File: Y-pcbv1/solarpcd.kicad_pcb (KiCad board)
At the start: 6 copper layers, 64 x 58 mm, 53 parts, among them IC2 TSL2561, J1 XF2M-1015-1A, J2 U.FL-R-SMT-1, J3 BATTERY CONNECTOR, U1 SWLP.12.B, U2 Value, U4 SW_SPDT

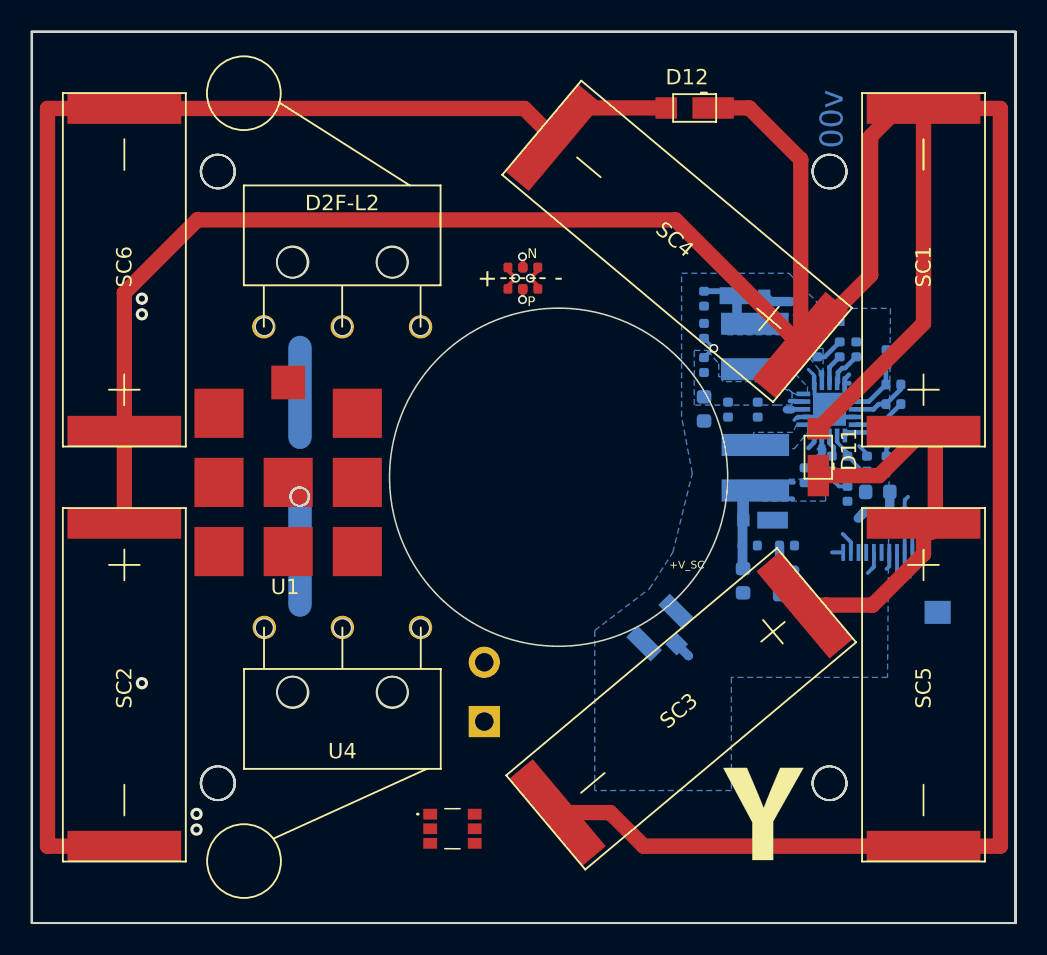
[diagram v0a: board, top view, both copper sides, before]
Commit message: Updated -Y PCB design
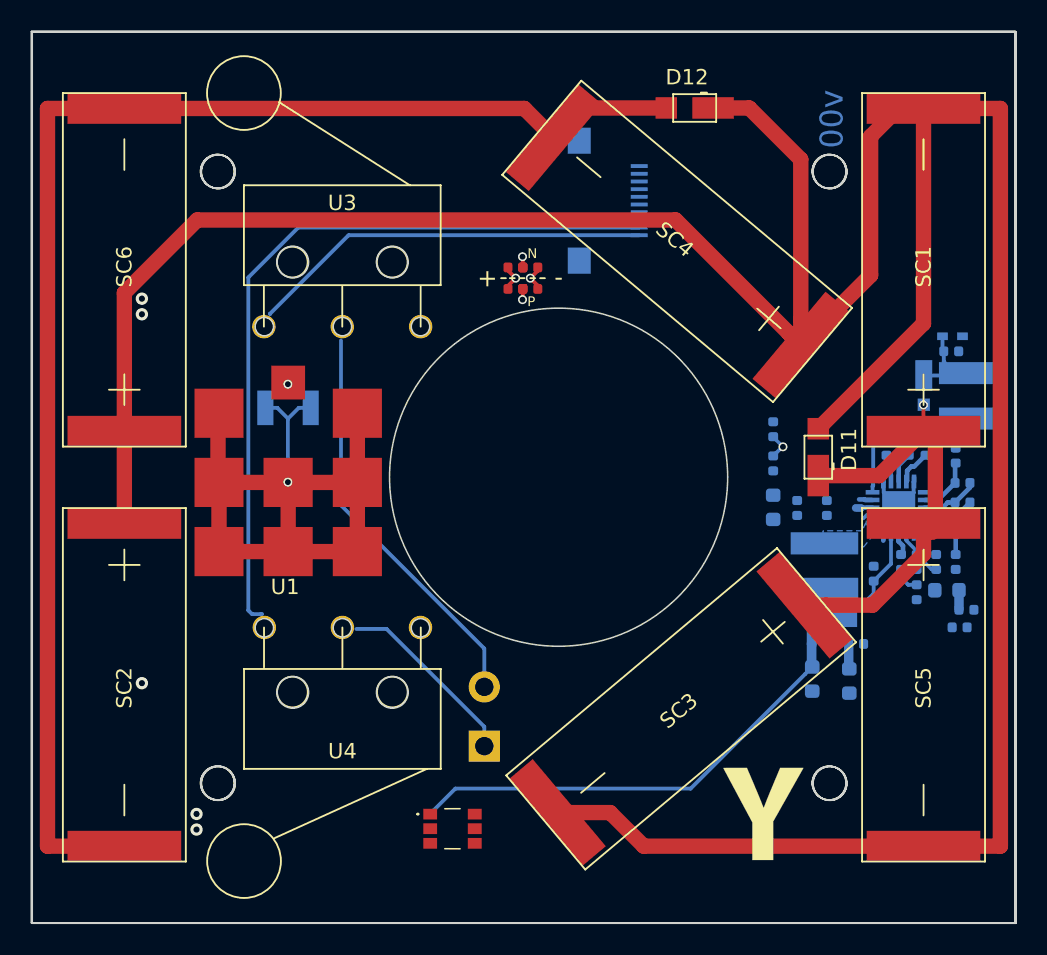
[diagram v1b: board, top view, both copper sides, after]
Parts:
- removed D2F-L2: D2F-L2-2, solarpcb:D2F-L2-2
- added U3: SW_SPDT, solarpcb:D2F-L2-2, F.Cu at (133.2, 89.2)
- D30: footprint custom-footprints:MICROSMP -> solarpcb:MICROSMP
- J1: footprint custom-footprints:XF2M-1015-1A -> solarpcb:XF2M-1015-1A
- U4: footprint custom-footprints:D2F-L2 -> solarpcb:D2F-L2
- moved J2 28.1 mm to (129.7, 94.5), turned to 0 degrees
- moved J1 27.7 mm to (152.5, 81.0), turned to 90 degrees
- moved C2 16.4 mm to (172.8, 90.8), turned to 0 degrees
- moved L1 14.5 mm to (174.2, 93.7)
- moved D30 13.0 mm to (171.0, 93.0), turned to 270 degrees
- moved D1 8.08 mm to (172.8, 89.8)
- moved C1 7.82 mm to (170.6, 106.5)
- moved C3 7.82 mm to (168.6, 97.1)
- moved C4 7.82 mm to (171.1, 97.1)
- moved C6 7.82 mm to (172.5, 106.3)
- moved D2 7.82 mm to (165.0, 108.2)
- moved L2 7.82 mm to (164.6, 104.8)
- moved R11 7.82 mm to (170.0, 97.1)
- moved R14 7.82 mm to (173.8, 107.6)
- moved R15 7.82 mm to (173.3, 108.8)
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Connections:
- IC2 pad 2: Net-(IC2-Pad2) -> (no net)
- IC2 pad 5: Net-(IC2-Pad5) -> (no net)
- J1 pad 5: BURN1 -> (no net)
- U4 pad 1: Net-(U4-Pad1) -> (no net)
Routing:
- net GND: track 116.8 -> 152.7 mm, vias 0 -> 1
- net +3V3: track 13.3 -> 46.9 mm
- net SCL1: track 30.8 -> 0.00 mm
- net BATT_P: track 55.7 -> 26.1 mm
- net SDA1: track 27.7 -> 0.00 mm
- net Net-(J3-Pad1): track 35.6 -> 12.7 mm
- net Net-(J3-Pad2): track 5.85 -> 26.4 mm
- net /VBAT: track 14.1 -> 2.40 mm
- net Net-(L1-Pad2): track 0.00 -> 10.8 mm
- net Net-(R11-Pad1): track 11.8 -> 3.79 mm
- net VOUT_EN: track 9.76 -> 1.74 mm
- net BATT_N: track 55.6 -> 49.4 mm
- net VSOLAR: track 6.82 -> 11.3 mm
- net Net-(R2-Pad2): track 7.46 -> 3.93 mm
- net COIL_N: track 31.4 -> 29.3 mm
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- removed copper zone on B.Cu, net +3V3
- removed copper zone on B.Cu, net GND
- removed copper zone on In3.Cu, net GND
- removed copper zone on B.Cu, net Net-(C11-Pad1)
- removed copper zone on B.Cu, net Net-(L1-Pad2)
- removed copper zone on B.Cu, net VSOLAR
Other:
- outline, holes or cut-outs redrawn
- board text removed: "+BATT"
- board text removed: "+V_SC"
- board text removed: "-BATT"
